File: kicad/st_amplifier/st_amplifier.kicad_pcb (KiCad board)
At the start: 2 copper layers, 170 x 80 mm, 80 parts

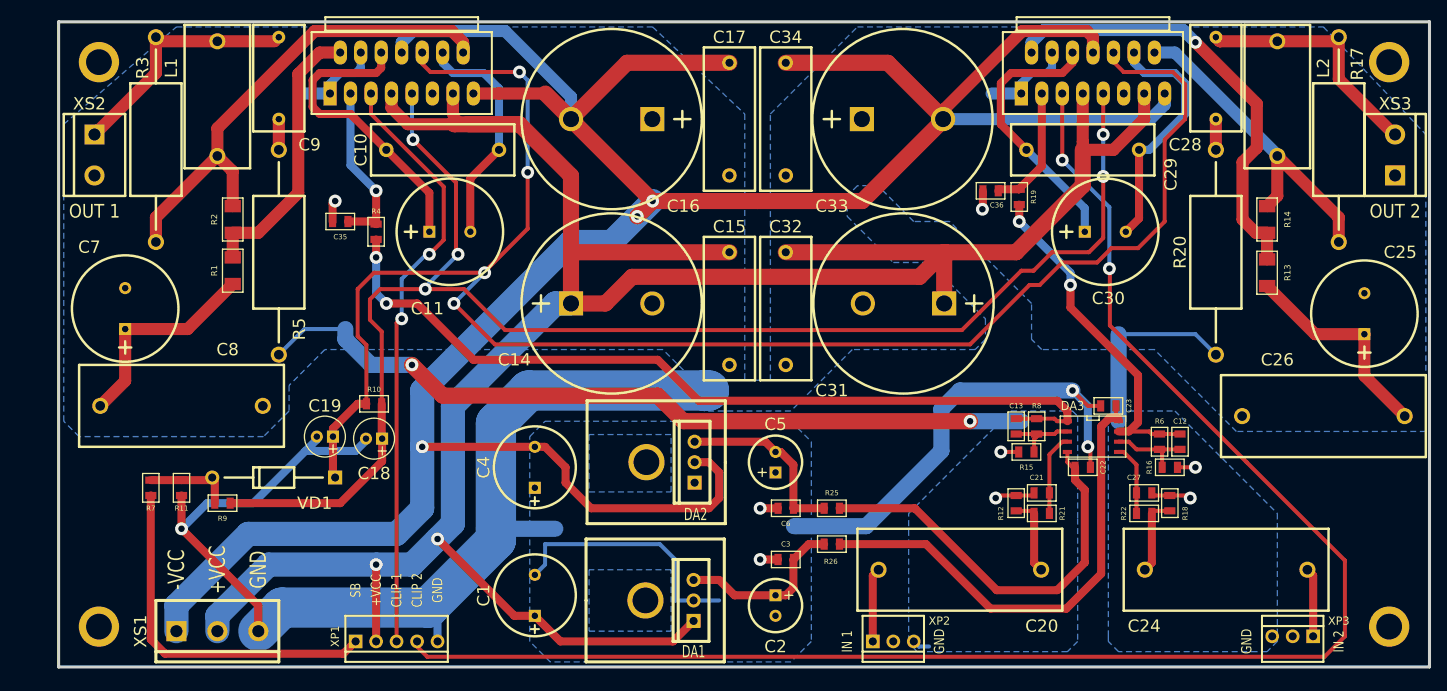
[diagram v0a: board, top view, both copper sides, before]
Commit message: New commit.
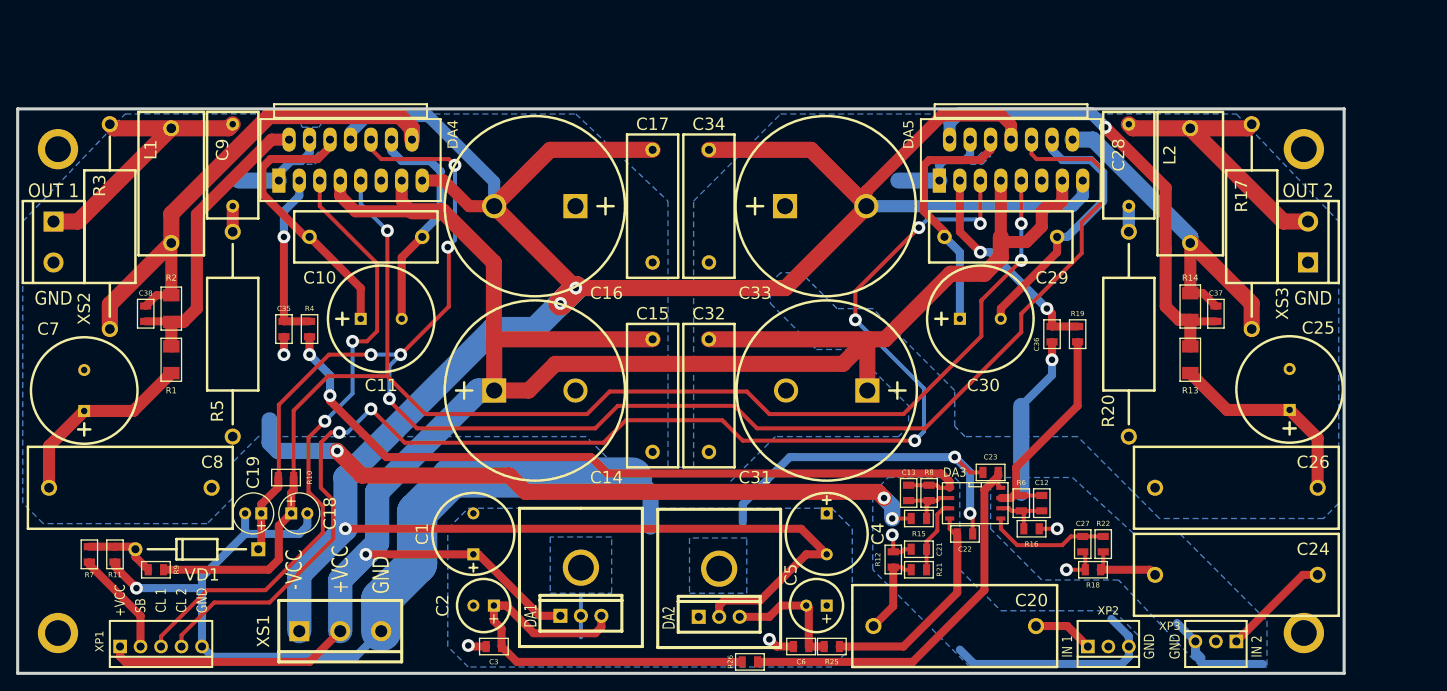
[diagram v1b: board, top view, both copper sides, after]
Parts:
- added C37: 22 п, SMD0805, F.Cu at (213.4, 85.1)
- added C38: 22 п, SMD0805, F.Cu at (80.6, 85.1)
- R14, R2: value 28.7 к +/-0.5% -> 28 к +/-0.5%
- R6, R8: value 22.1 к +/-0.5% -> 24 к +/-0.5%
- moved C3 37.8 mm to (123.8, 126.4)
- moved C4 37.1 mm to (165.1, 112.4), turned to 270 degrees
- moved C2 36.2 mm to (122.6, 121.3), turned to 180 degrees
- moved XP1 29.2 mm to (82.5, 126.4)
- moved XP2 26.7 mm to (200.0, 126.4)
- moved DA2 19.4 mm to (151.8, 122.7), turned to 90 degrees
- moved C36 19.3 mm to (193.0, 87.6), turned to 270 degrees
- moved C30 18.9 mm to (184.2, 85.7)
- moved R16 18.8 mm to (190.5, 111.8)
- moved R6 18.8 mm to (189.2, 108.6)
- moved C12 18.8 mm to (191.8, 108.6)
- moved R19 18.5 mm to (196.2, 87.6)
- moved C5 18.5 mm to (163.8, 121.3), turned to 180 degrees
- moved 1_PIN 18.1 mm to (153.3, 116.7), turned to 90 degrees
- moved R26 17.8 mm to (155.6, 128.3)
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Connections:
- XP1 pad 1: /MU/ST -> /+29V
- XP1 pad 2: /+29V -> /MU/ST
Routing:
- net /GND: track 403.2 -> 364.0 mm
- net /CLIP_2: track 199.1 -> 164.3 mm, vias 2 -> 6
- net /+29V: track 313.5 -> 280.7 mm, vias 2 -> 1
- net /MU/ST: track 44.6 -> 13.1 mm
- net /+15V: track 21.7 -> 52.3 mm
- net N-0000022: track 50.8 -> 27.2 mm
- net N-000005: track 43.7 -> 28.0 mm, vias 2 -> 0
- net N-0000021: track 60.8 -> 48.8 mm
- net /MUTE: track 215.5 -> 204.4 mm, vias 4 -> 5
- net N-0000011: track 15.8 -> 26.8 mm, vias 0 -> 2
- net N-000002: track 106.2 -> 96.0 mm
- net /STBY: track 186.2 -> 176.0 mm, vias 5 -> 3
- net /-15V: track 22.6 -> 16.0 mm
- net /-29V: track 342.9 -> 336.4 mm
- net N-000003: track 8.91 -> 15.3 mm
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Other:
- board size 170 x 80 mm -> 164.5 x 70 mm
- board text added: "CL 1"
- board text added: "CL 2"
- board text removed: "CLIP 1"
- board text removed: "CLIP 2"
